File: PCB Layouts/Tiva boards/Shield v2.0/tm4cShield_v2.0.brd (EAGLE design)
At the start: 51.7 x 31.7 mm, 14 parts

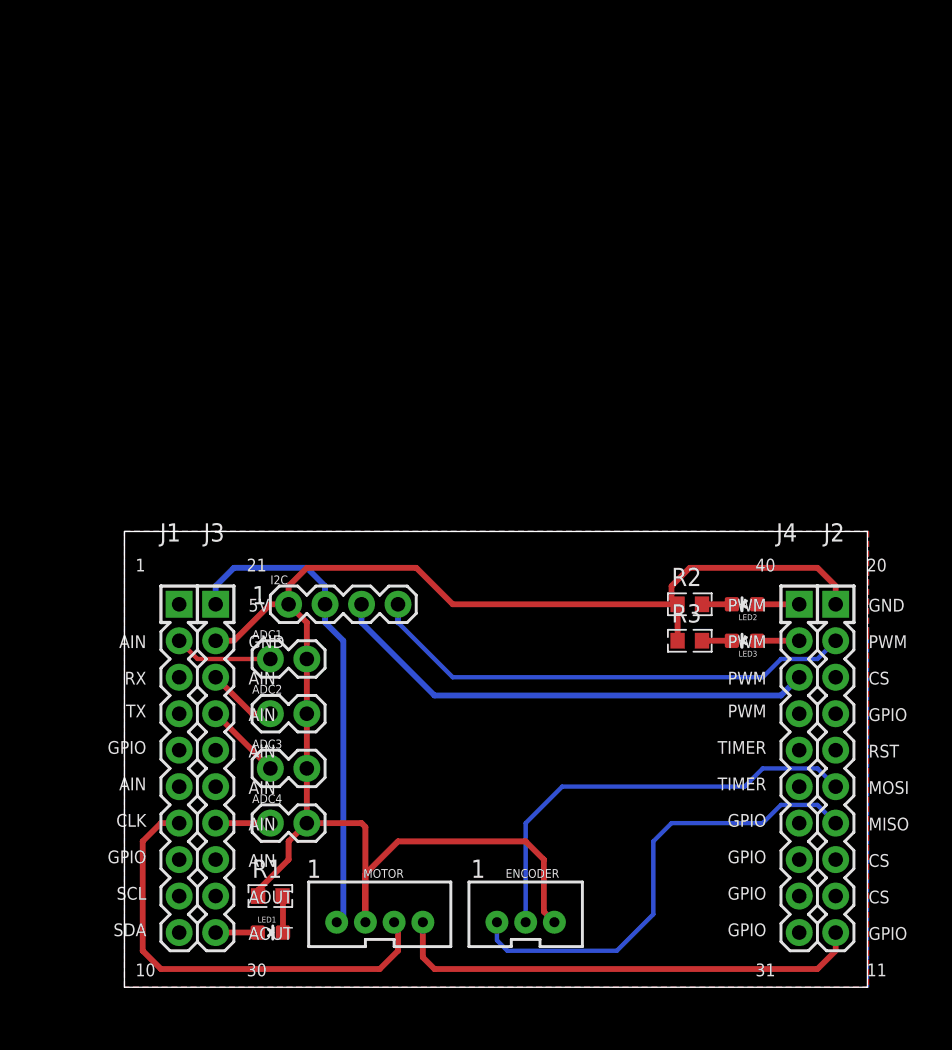
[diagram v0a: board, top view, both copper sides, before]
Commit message: Tiva shield
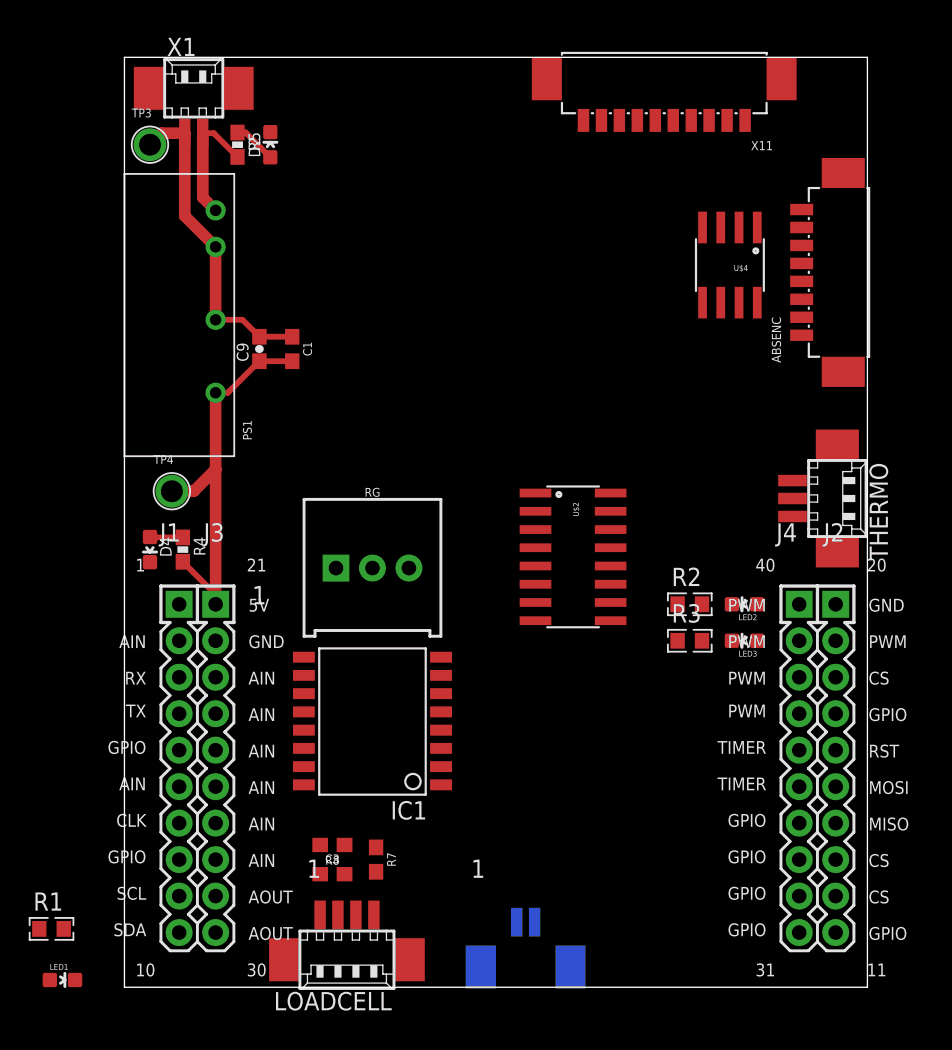
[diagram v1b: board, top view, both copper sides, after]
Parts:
- removed ADC1, ADC3, ADC4: (no value), SparkFun-Connectors:1X02
- removed ENCODER: (no value), SparkFun-Connectors:JST-3-PTH-VERT
- removed I2C: (no value), SparkFun-Connectors:1X04
- removed MOTOR: (no value), SparkFun-Connectors:JST-4-PTH-VERT
- added ABSENC: x5, pel_molex:PB-53261-08
- added C1, C3: 0.1uF, SparkFun-Capacitors:0603
- added C9: 2.2u, test_Beast_Elmo_Twitter_Carrier_Board_V1:0603-CAP
- added D2: 12V, test_Beast_Elmo_Twitter_Carrier_Board_V1:LED-0603
- added D4: 5V, test_Beast_Elmo_Twitter_Carrier_Board_V1:LED-0603
- added IC1: INA125U, burr-brown:SO16-1
- added LOADCELL: x2, con-molex:53261-04
- added PS1: 12/5, murata-supplys:MURATA_NMG
- added R4: 1k, test_Beast_Elmo_Twitter_Carrier_Board_V1:0603-RES
- added R5: 4k7, test_Beast_Elmo_Twitter_Carrier_Board_V1:0603-RES
- added R7, R8: 10k, SparkFun-Resistors:0603
- added RG: 10k, SparkFun-Resistors:TRIMPOT-PTH-3386U
- added THERMO: x4, con-molex:53261-03
- added TP3: GND, testpad:5000_SERIES_TESTPOINT
- added TP4: 5V, testpad:5000_SERIES_TESTPOINT
- added U$2: SN75175, RoMeLa:SOIC16
- added U$4: SP490, RoMeLa:SOIC8
- added X1: x1, con-molex:53261-02
- added X11: (no value), pel_molex:PB-53261-10
- ADC2: value (none) -> x3; device SparkFun-Connectors:1X02 -> con-molex:53261-02
- moved ADC2 24.6 mm to (47.0, 23.6), flipped to the bottom, turned to 180 degrees
- moved R1 15.4 mm to (14.0, 25.7)
- moved LED1 14.8 mm to (14.7, 22.1)
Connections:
- net N$11 renamed PA5
- net N$12 renamed PA6
- net N$13 renamed PA7
- net N$18 renamed PD2
- net N$19 renamed PD3
- net N$30 renamed PC7
- net N$31 renamed PD6
- net N$32 renamed PD7
- net N$33 renamed PF4
- net N$37 renamed PF0
- net N$38 renamed RST
- net N$4 renamed PB0
- net N$42 renamed PA3
- net N$5 renamed PB1
- net N$8 renamed PE4
- net N$9 renamed PE5
- removed net N$22: A1.29
- removed net N$27: A1.37
- removed net N$28: A1.36
- removed net N$29: A1.35
- removed net N$36: A1.18
- removed net N$41: A1.13
- new net CASE: ABSENC.7
- new net CH_A: U$2.2, X11.6
- new net CH_A*: U$2.1, X11.5
- new net CH_B: U$2.6, X11.8
- new net CH_B*: U$2.7, X11.7
- new net CH_I: U$2.10, X11.10
- new net CH_I*: U$2.9, X11.9
- new net CLOCK+: ABSENC.2, U$4.5
- new net CLOCK-: ABSENC.3, U$4.6
- new net DATA+: ABSENC.4, U$4.8
- new net DATA-: ABSENC.5, U$4.7
- new net N$1: D4.A, R4.1
- new net N$10: IC1.9, RG.2
- new net N$14: A1.20
- new net N$17: U$2.13
- new net N$20: U$2.14
- new net N$3: IC1.8, RG.1
- new net N$35: D2.A, R5.1
- new net N$9: ABSENC.6
- new net PA4: A1.13, U$4.2
- new net PC4: A1.37, U$2.11
- new net PC5: A1.36, U$2.3
- new net PC6: A1.35, U$2.5
- new net PE0: A1.18, THERMO.2
- new net PE2: A1.28, ADC2.1
- new net PE3: A1.29, IC1.10, IC1.11
- new net V+: LOADCELL.3
- new net V-: IC1.7, LOADCELL.2, R7.2
- new net VIN: C3.2, IC1.1, IC1.2, IC1.6, PS1.VIN+, R5.2, R8.1, X1.1
- new net V_2.5: IC1.14, IC1.4, IC1.5, LOADCELL.4
- net 5V: now also ABSENC.1, C1.2, C9.1, PS1.VOUT+, R4.2, THERMO.1, TP4.P$1, U$2.12, U$2.16, U$2.4, U$4.1, X11.2; no longer I2C.2, MOTOR.1
- net GND: now also ABSENC.8, C1.1, C3.1, C9.2, D2.C, D4.C, IC1.12, IC1.3, LOADCELL.1, PS1.VIN-, PS1.VOUT-, R7.1, R8.2, THERMO.3, TP3.P$1, U$2.8, U$4.4, X1.2, X11.3; no longer A1.20, ADC1.2, ADC3.2, ADC4.2, ENCODER.3, I2C.1, MOTOR.2, R1.1, R2.1, R3.1
- net N$21: now also U$2.15; no longer A1.28
- net PA2: now also U$4.3; no longer MOTOR.4
- net PB2: no longer I2C.4
- net PB3: no longer I2C.3
- net PB4: no longer MOTOR.3
- net PB5: no longer ADC1.1
- net PB6: no longer ENCODER.1
- net PB7: no longer ENCODER.2
- net PD0: no longer ADC2.1
- net PD1: no longer ADC3.1
- net PE1: no longer ADC4.1
- net PF1: no longer LED1.A
- net PF2: no longer LED2.A
- net PF3: no longer LED3.A
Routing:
- net GND: track 108.8 -> 22.5 mm
- net PB3: track 34.4 -> 0.00 mm
- net PB2: track 34.4 -> 0.00 mm
- net PA2: track 33.3 -> 0.00 mm
- net PB6: track 32.9 -> 0.00 mm
- net PB4: track 31.6 -> 0.00 mm
- net PB7: track 30.6 -> 0.00 mm
- net VIN: track 0.00 -> 8.85 mm
- net PB5: track 6.88 -> 0.00 mm
- net PD1: track 5.39 -> 0.00 mm
- net PD0: track 4.86 -> 0.00 mm
- net 5V: track 34.1 -> 29.6 mm
- net PE1: track 3.81 -> 0.00 mm
- net N$35: track 0.00 -> 3.00 mm
- net PF3: track 2.93 -> 0.00 mm
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- removed copper zone on layer 1, net GND
- removed copper zone on layer 16, net GND
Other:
- board size 51.7 x 31.7 mm -> 51.7 x 64.8 mm
